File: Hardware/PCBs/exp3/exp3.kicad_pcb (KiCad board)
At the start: 2 copper layers, 52.1 x 35.6 mm, 8 parts, among them J1 Conn_01x07_Female, J2 Conn_01x06_Female, U1 74HC86, U2 7483

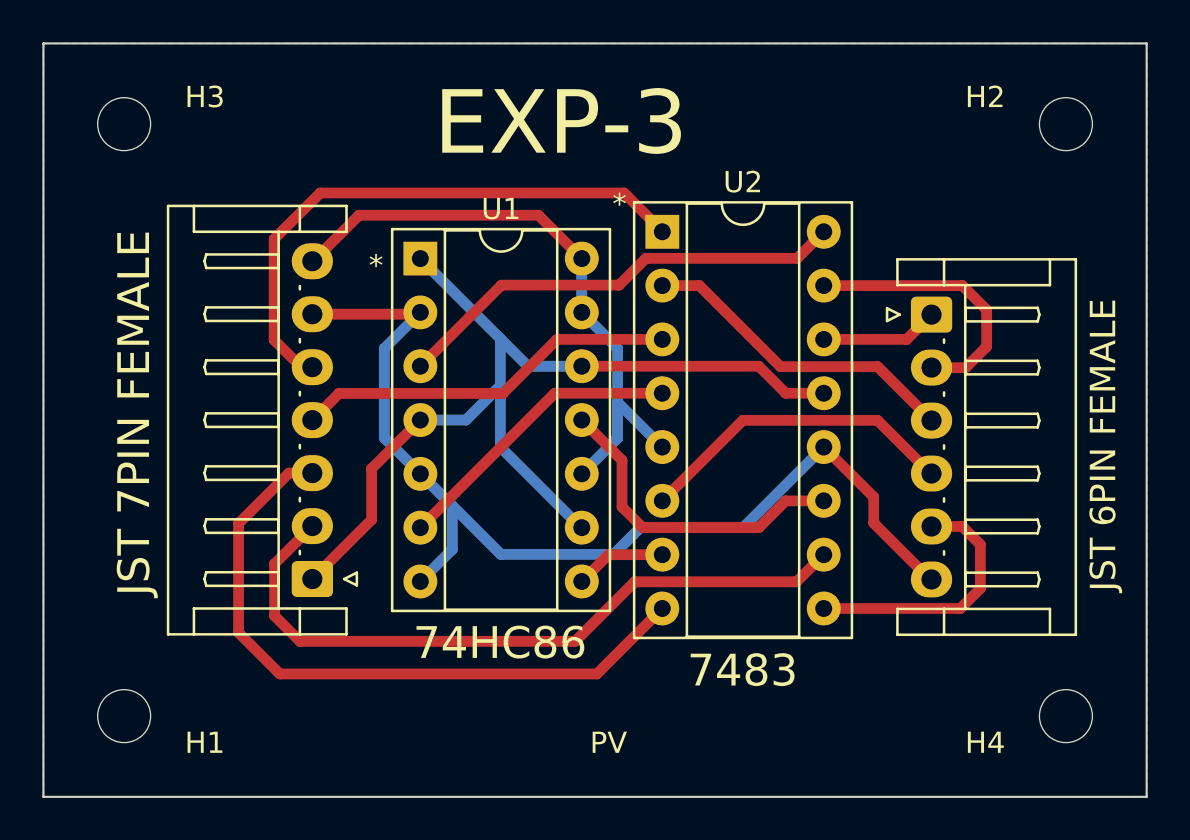
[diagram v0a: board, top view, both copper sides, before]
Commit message: Exp - 2 and 3 PCB Updated
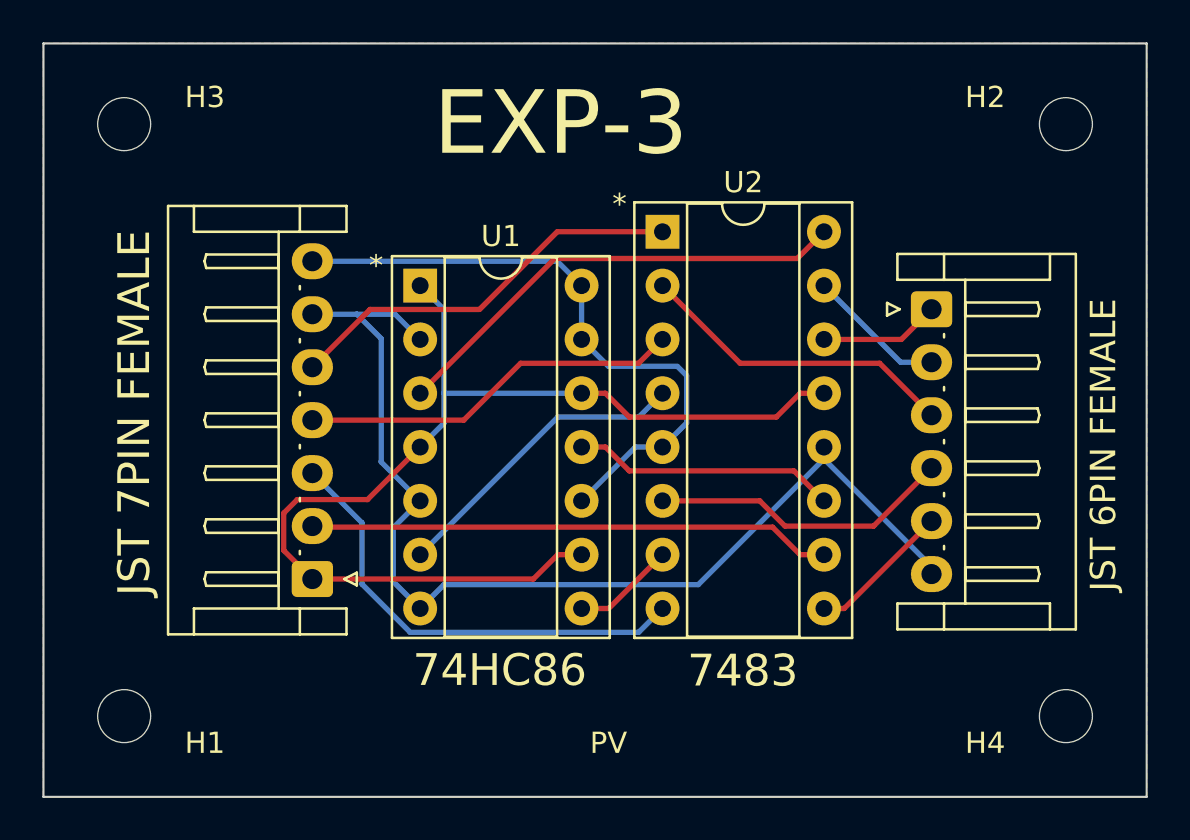
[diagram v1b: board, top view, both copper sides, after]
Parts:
- moved U1 1.28 mm to (124.5, 88.9)
- moved J2 0.25 mm to (148.6, 90.0)
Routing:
- net A1: track 31.7 -> 21.8 mm
- net A0: track 33.1 -> 24.7 mm
- net A3: track 27.1 -> 19.2 mm
- net S3: track 12.9 -> 6.58 mm
- net Cin: track 46.2 -> 52.0 mm
- net S0: track 12.5 -> 6.79 mm
- net Net-(U1-Pad11): track 15.3 -> 12.5 mm
- net GND: track 49.4 -> 51.8 mm
- net S1: track 15.3 -> 14.3 mm
- net VCC: track 30.7 -> 30.1 mm
- net Net-(U1-Pad3): track 21.7 -> 22.2 mm
- net Net-(U1-Pad8): track 4.32 -> 4.87 mm
- net Net-(U1-Pad6): track 14.0 -> 14.6 mm
